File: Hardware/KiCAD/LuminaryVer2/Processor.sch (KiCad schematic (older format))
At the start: 18 parts, among them SW1 SW_Push, U2 STM32L432KBUx, U6 AT25SF081-SSHD-X

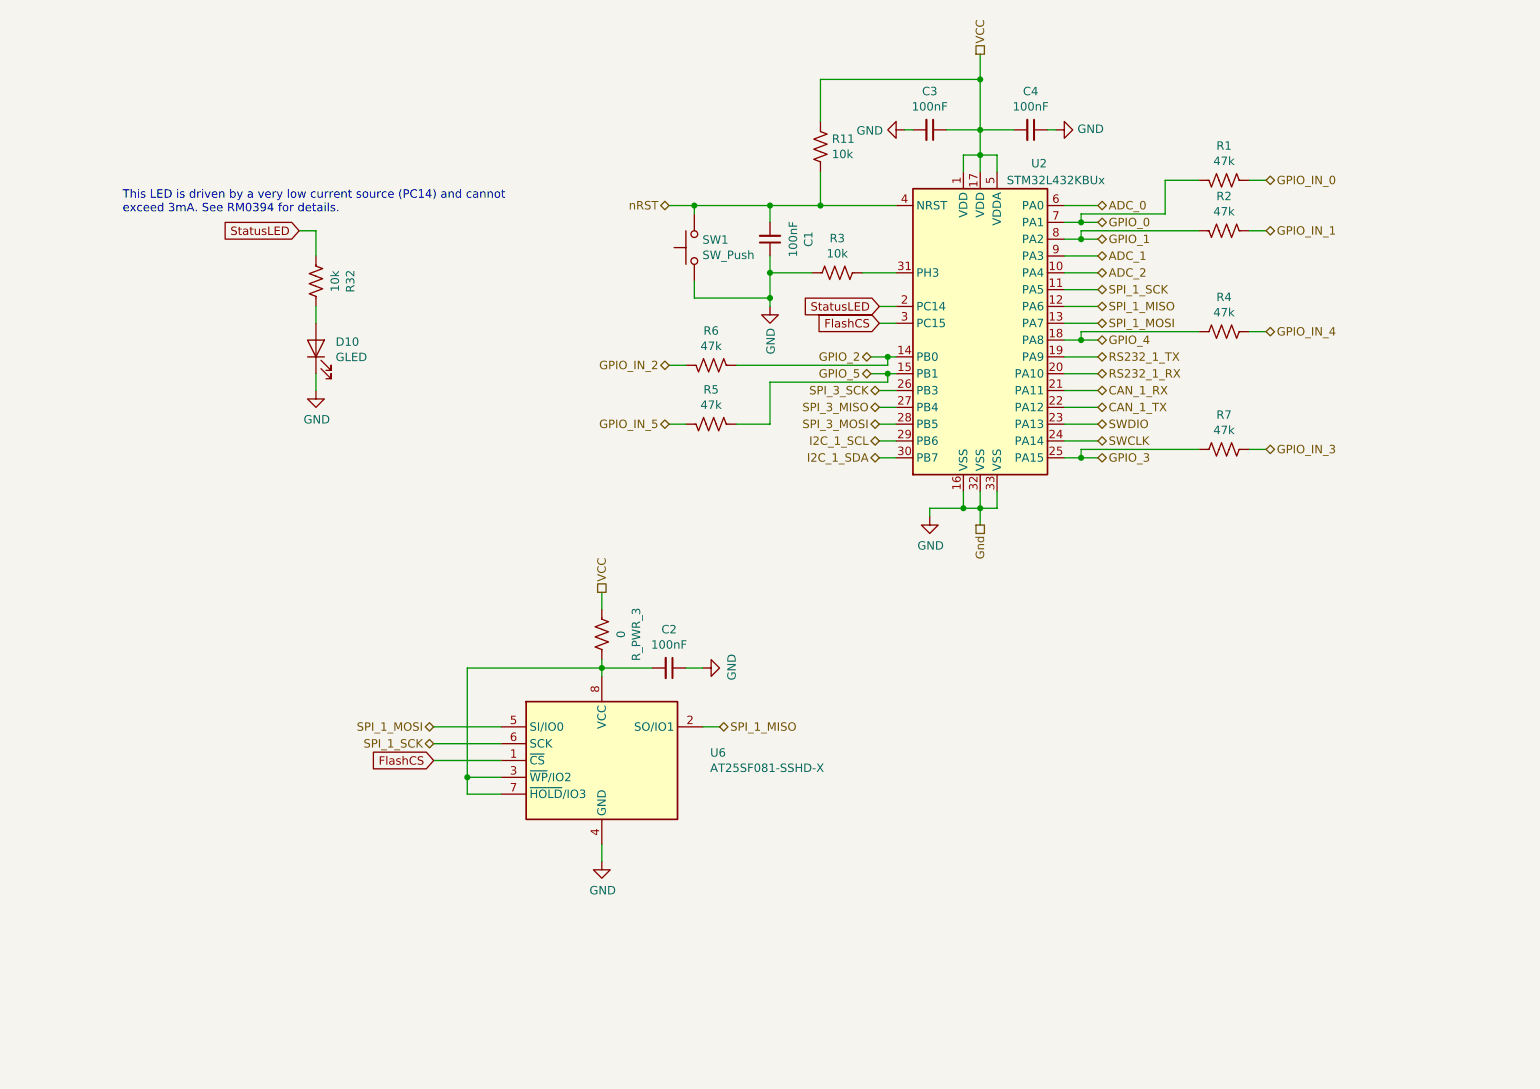
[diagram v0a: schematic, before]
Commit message: Updated version 2 hardware schematics.
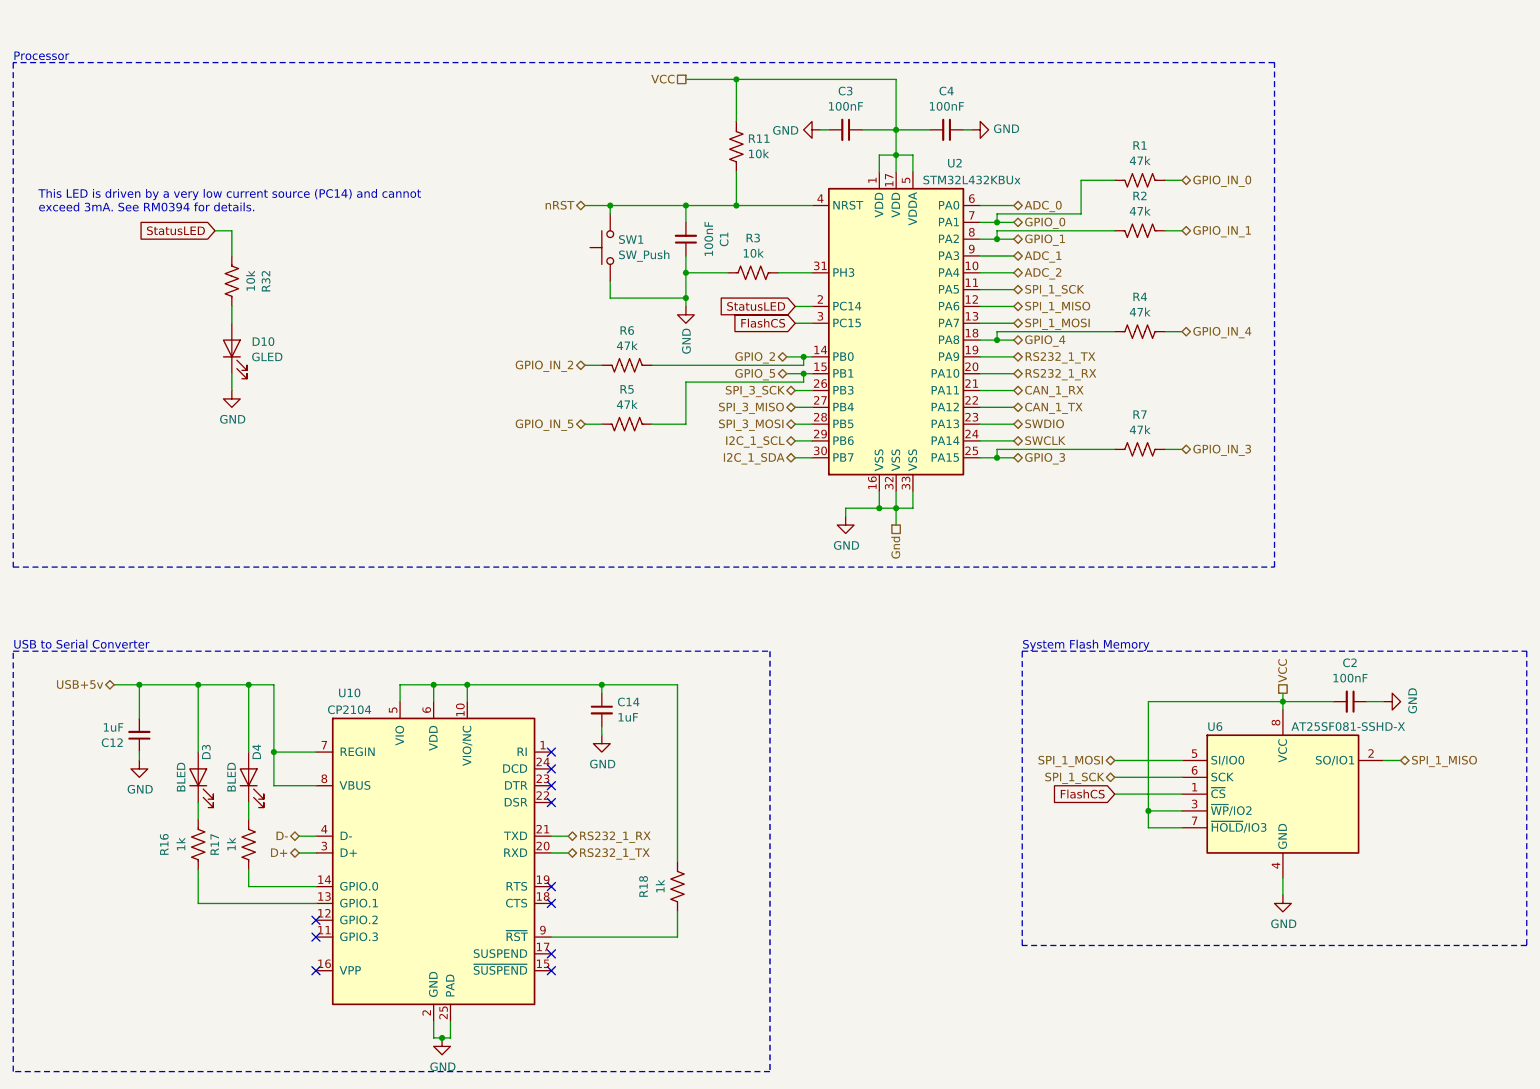
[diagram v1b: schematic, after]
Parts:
- removed R_PWR_3: 0, Resistor_SMD:R_0402_1005Metric, symbol Device:R_US
- added C12, C14: 1uF, Capacitor_SMD:C_0805_2012Metric, symbol Device:C_Small
- added D3, D4: BLED, Diode_SMD:D_0603_1608Metric, symbol Device:LED
- added R16, R17, R18: 1k, Resistor_SMD:R_0402_1005Metric, symbol Device:R_US
- added U10: CP2104, Package_DFN_QFN:QFN-24-1EP_4x4mm_P0.5mm_EP2.6x2.6mm, symbol Interface_USB:CP2104
- D10: LCSC C205443 -> C72043; PartNumber ORH-G36G -> 19-217/GHC-YR1S2/3T
- R11, R3, R32: LCSC C102759 -> C25744
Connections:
- net GND: now also C12.1, C14.2, U10.2 (GND), U10.25 (PAD)
- net RS232_1_RX: now also U10.21 (TXD)
- net RS232_1_TX: now also U10.20 (RXD)
- net VCC: now also C2.2, U6.3 (~WP~/IO2), U6.7 (~HOLD~/IO3), U6.8 (VCC)
- new net: C14.1, R18.2, U10.10 (VIO/NC), U10.5 (VIO), U10.6 (VDD)
- new net: R16.1, U10.13 (GPIO.1)
- new net: R17.1, U10.14 (GPIO.0)
- new net: R18.1, U10.9 (~RST)
- new net: D4.1 (K), R17.2
- new net: D3.1 (K), R16.2
- new net D+: U10.3 (D+)
- new net D-: U10.4 (D-)
- new net USB+5v: C12.2, D3.2 (A), D4.2 (A), U10.7 (REGIN), U10.8 (VBUS)
- no-connect marks 0 -> 11
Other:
- note added: "Processor"
- note added: "System Flash Memory"
- note added: "USB to Serial Converter"
- moved on the sheet: C1, C2, C3, C4, D10, R1, R11, R2, R3, R32, R4, R5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
